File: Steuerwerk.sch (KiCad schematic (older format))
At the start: 134 parts, among them P1 CONN_01X01, P10 CONN_01X01, P11 CONN_01X01, P12 CONN_01X01, P13 CONN_01X01, P14 CONN_01X01, P15 CONN_01X01, P16 CONN_01X01, P17 CONN_01X01, P18 CONN_01X01, P19 CONN_01X01, P2 CONN_01X01, P20 CONN_01X01, P21 CONN_01X01, P22 CONN_01X01, P23 CONN_01X01, P24 CONN_01X01, P3 CONN_01X01, P4 CONN_01X01, P5 CONN_01X01, P6 CONN_01X01, P7 CONN_01X01, P8 CONN_01X01, P9 CONN_01X01, Q1 Q_PNP_BCE, U1 74LS04, U2 74LS161, U3 74LS04, U4 74LS138, U5 74LS138, U6 74LS04, U7 74LS374, U8 74LS04, U9 74LS374

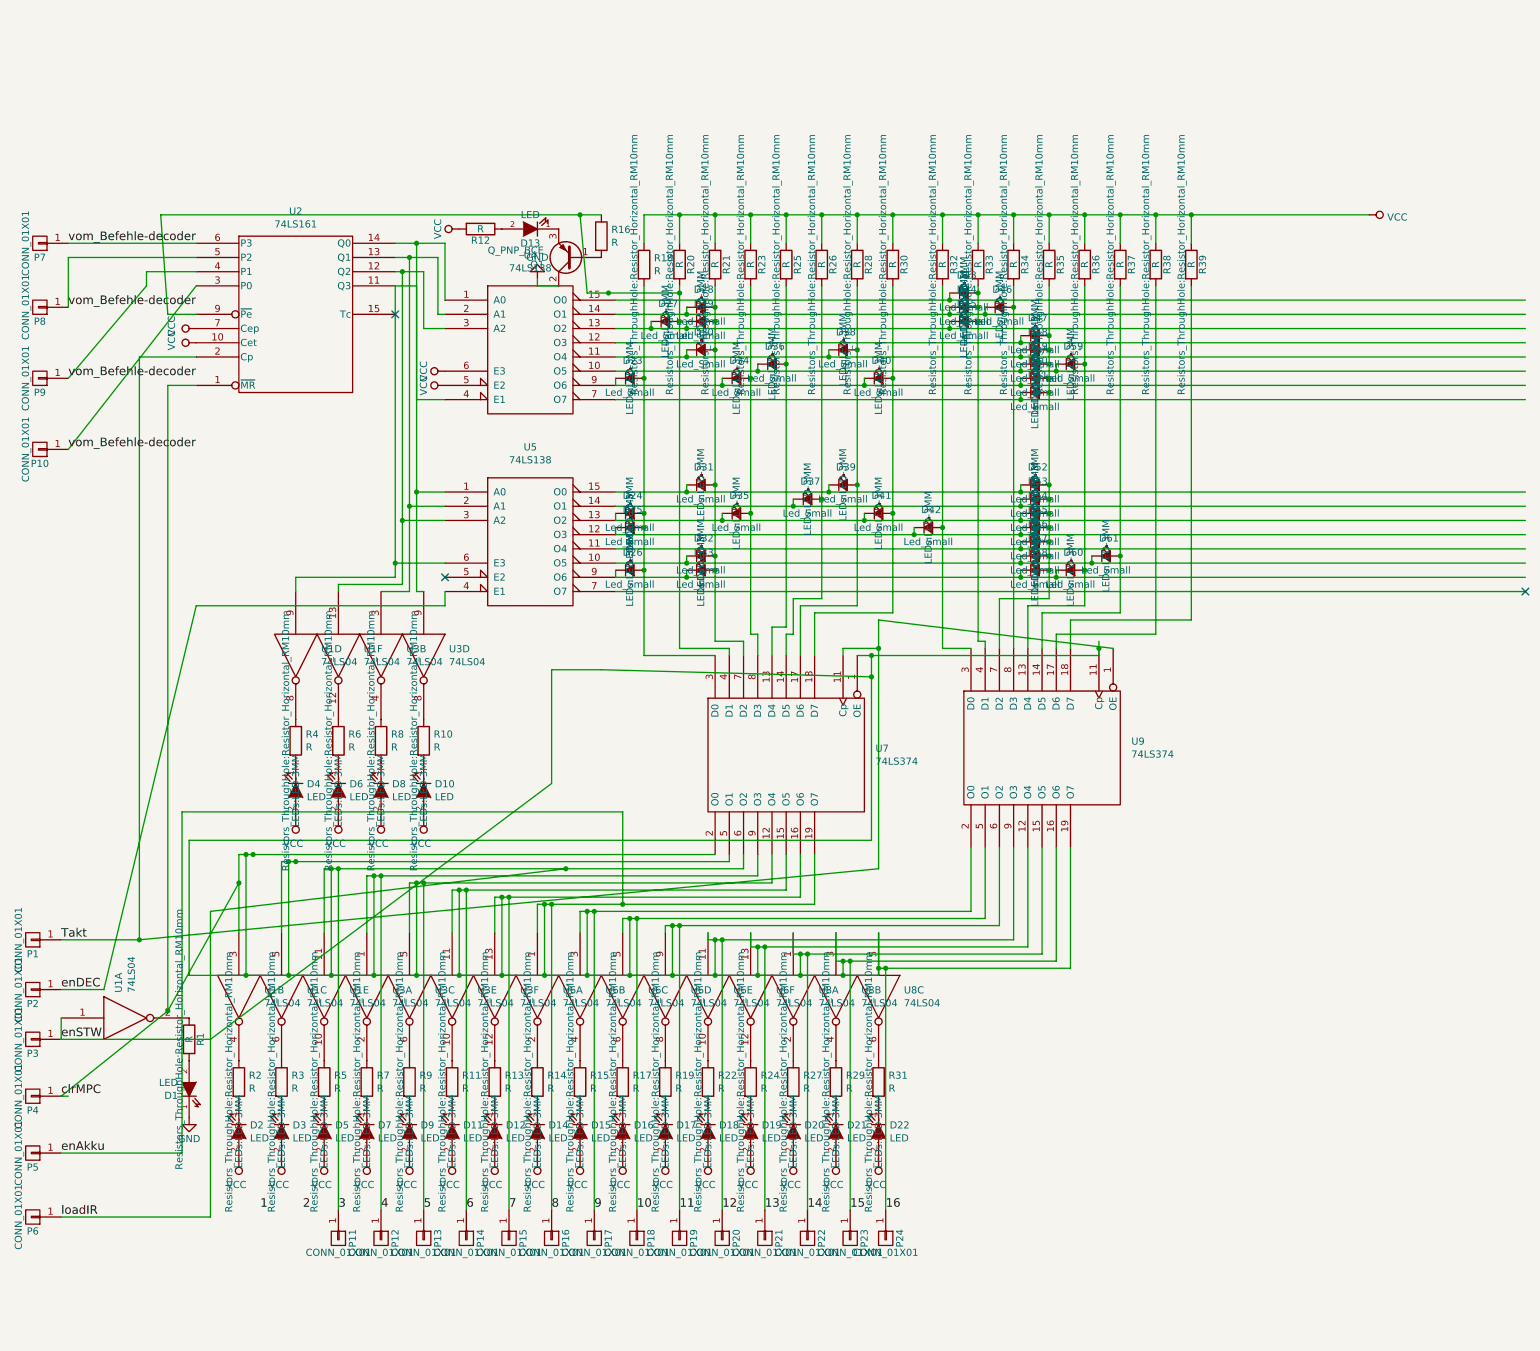
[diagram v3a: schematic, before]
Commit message: neue Steuerwerk Resistoren mit dateien
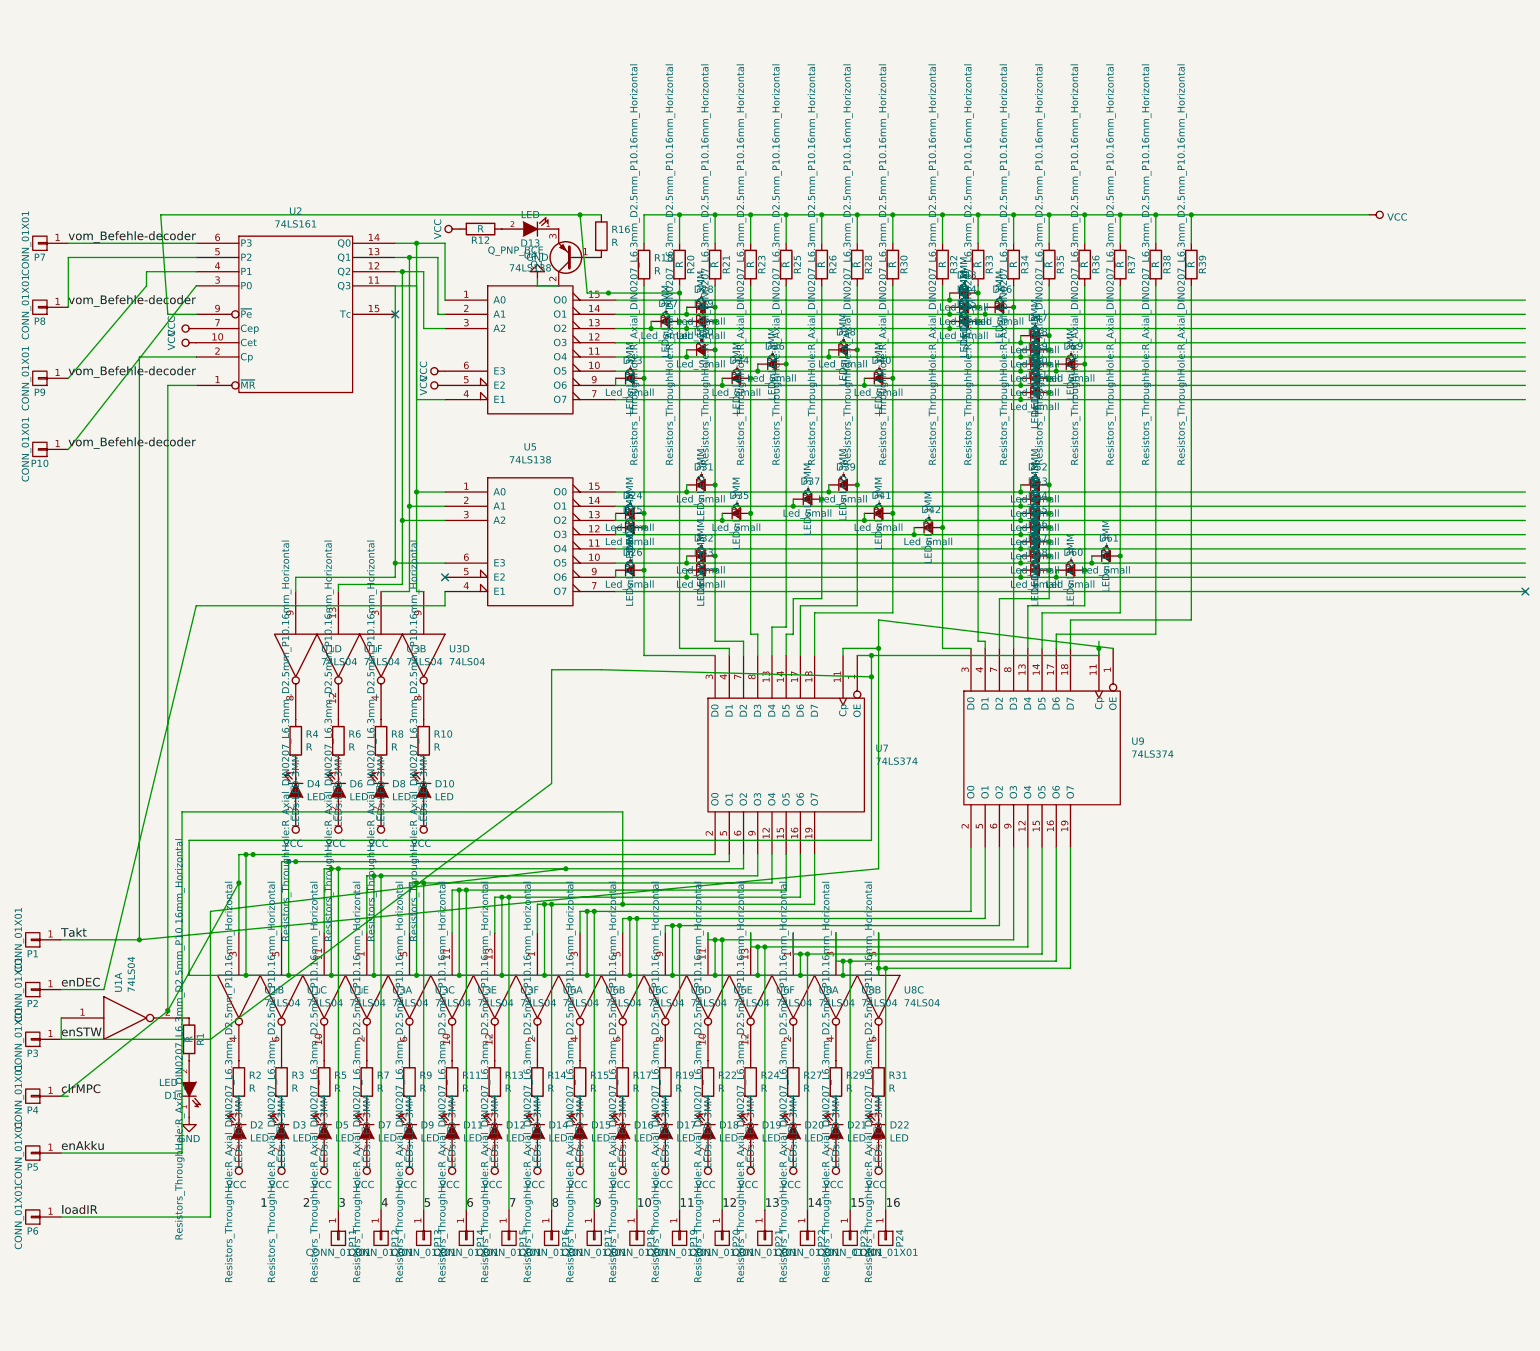
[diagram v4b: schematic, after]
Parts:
- R1, R10, R11, R12, R13, R14, R15, R17, R18, R19, R2, R20, R21, R22, R23, R24, R25, R26, R27, R28, R29, R3, R30, R31, R32, R33, R34, R35, R36, R37, R38, R39, R4, R5, R6, R7, R8, R9: footprint Resistors_ThroughHole:Resistor_Horizontal_RM10mm -> Resistors_ThroughHole:R_Axial_DIN0207_L6.3mm_D2.5mm_P10.16mm_Horizontal

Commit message: Dioden und Anschlüsse
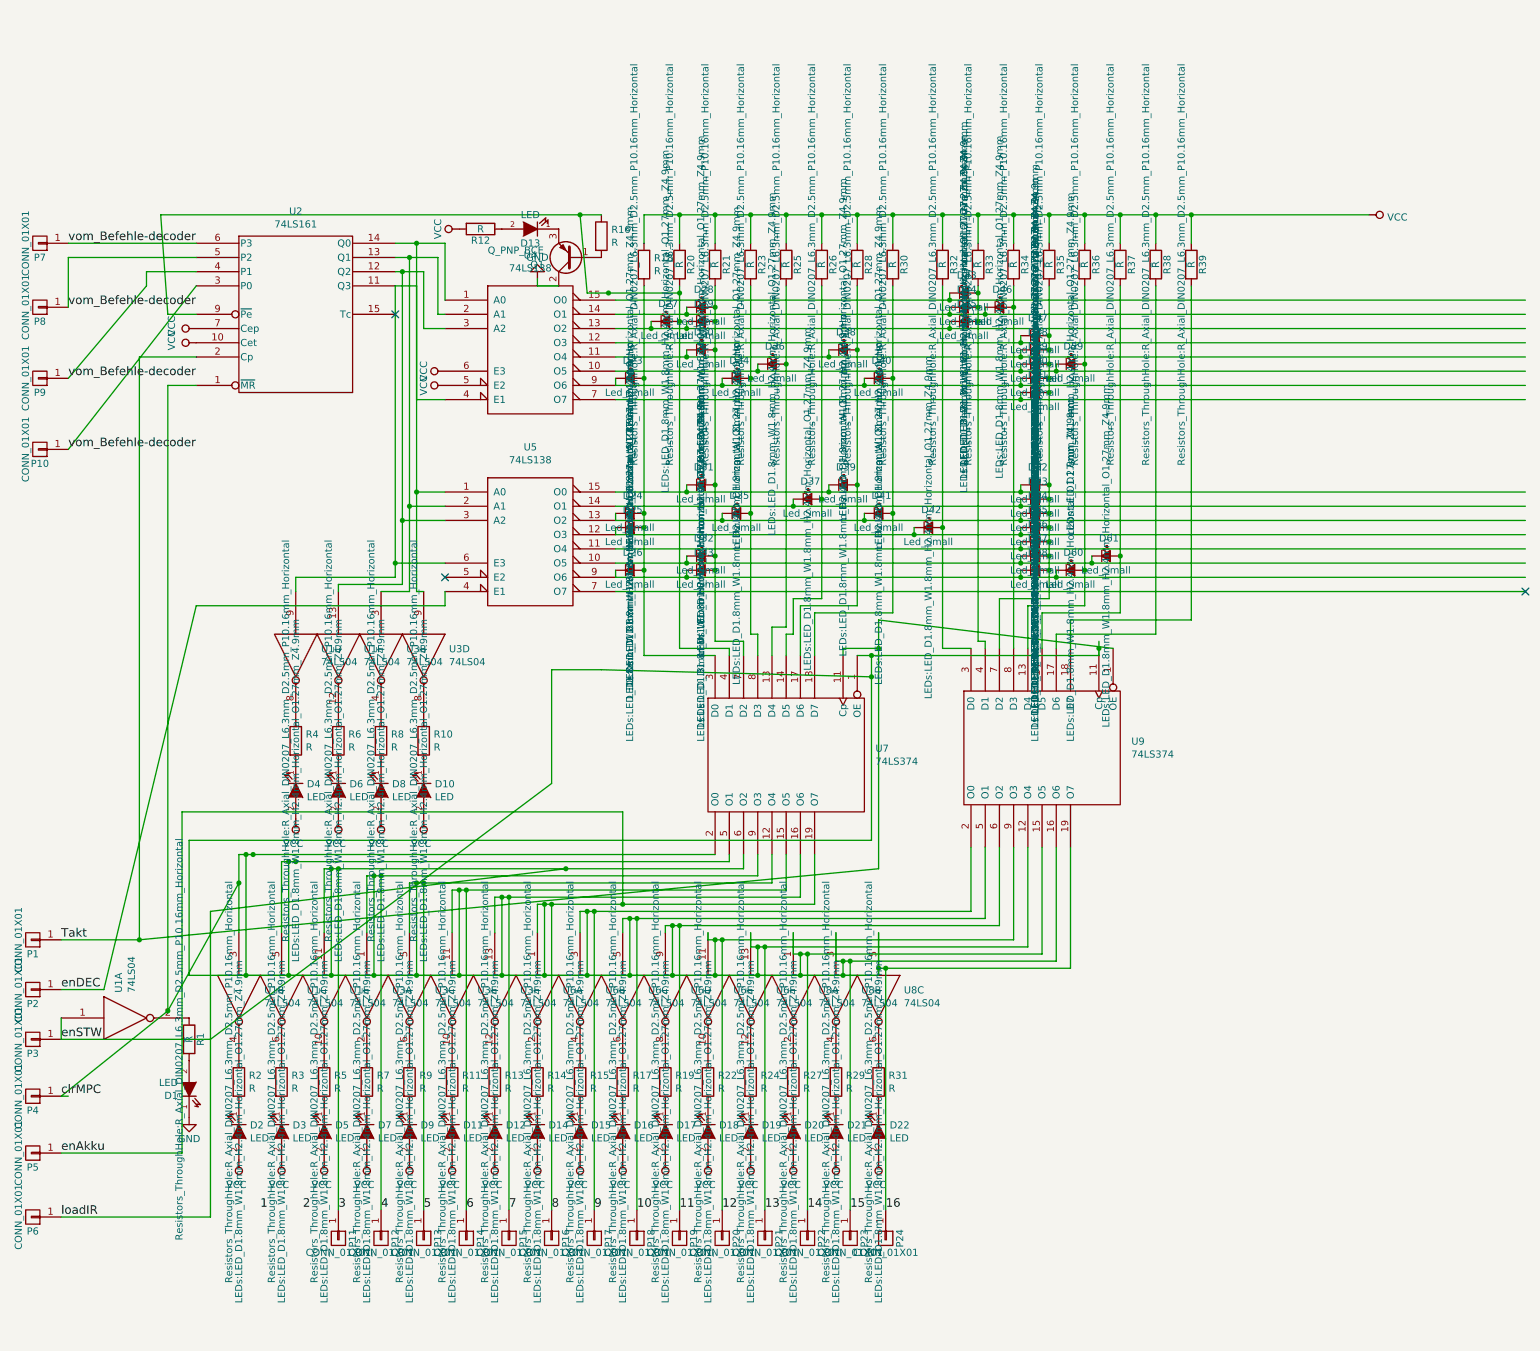
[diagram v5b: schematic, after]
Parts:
- D1, D30: footprint (none) -> LEDs:LED_D1.8mm_W1.8mm_H2.4mm_Horizontal_O1.27mm_Z4.9mm
- D10, D11, D12, D13, D14, D15, D16, D17, D18, D19, D2, D20, D21, D22, D23, D24, D25, D26, D27, D28, D3, D31, D32, D33, D34, D35, D36, D37, D38, D39, D4, D40, D41, D42, D43, D44, D45, D46, D47, D48, D49, D5, D50, D51, D52, D53, D54, D55, D56, D57, D58, D59, D6, D60, D61, D7, D8, D9: footprint LEDs:LED-3MM -> LEDs:LED_D1.8mm_W1.8mm_H2.4mm_Horizontal_O1.27mm_Z4.9mm
- P1, P11, P12, P13, P14, P15, P16, P17, P18, P19, P2, P20, P21, P22, P23, P24, P3, P4, P5, P6, P7, P8, P9: footprint (none) -> Connect:1pin
